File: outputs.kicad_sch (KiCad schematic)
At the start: 33 parts, among them J12 Water_Pump, J13 Fan_Continous, J2 mist, J3 Led, J8 Fan_Exhaust, Q1 AO3406, Q2 AO3406, Q3 AO3406, Q4 AO3406, Q5 AO3406, Q6 AO3406

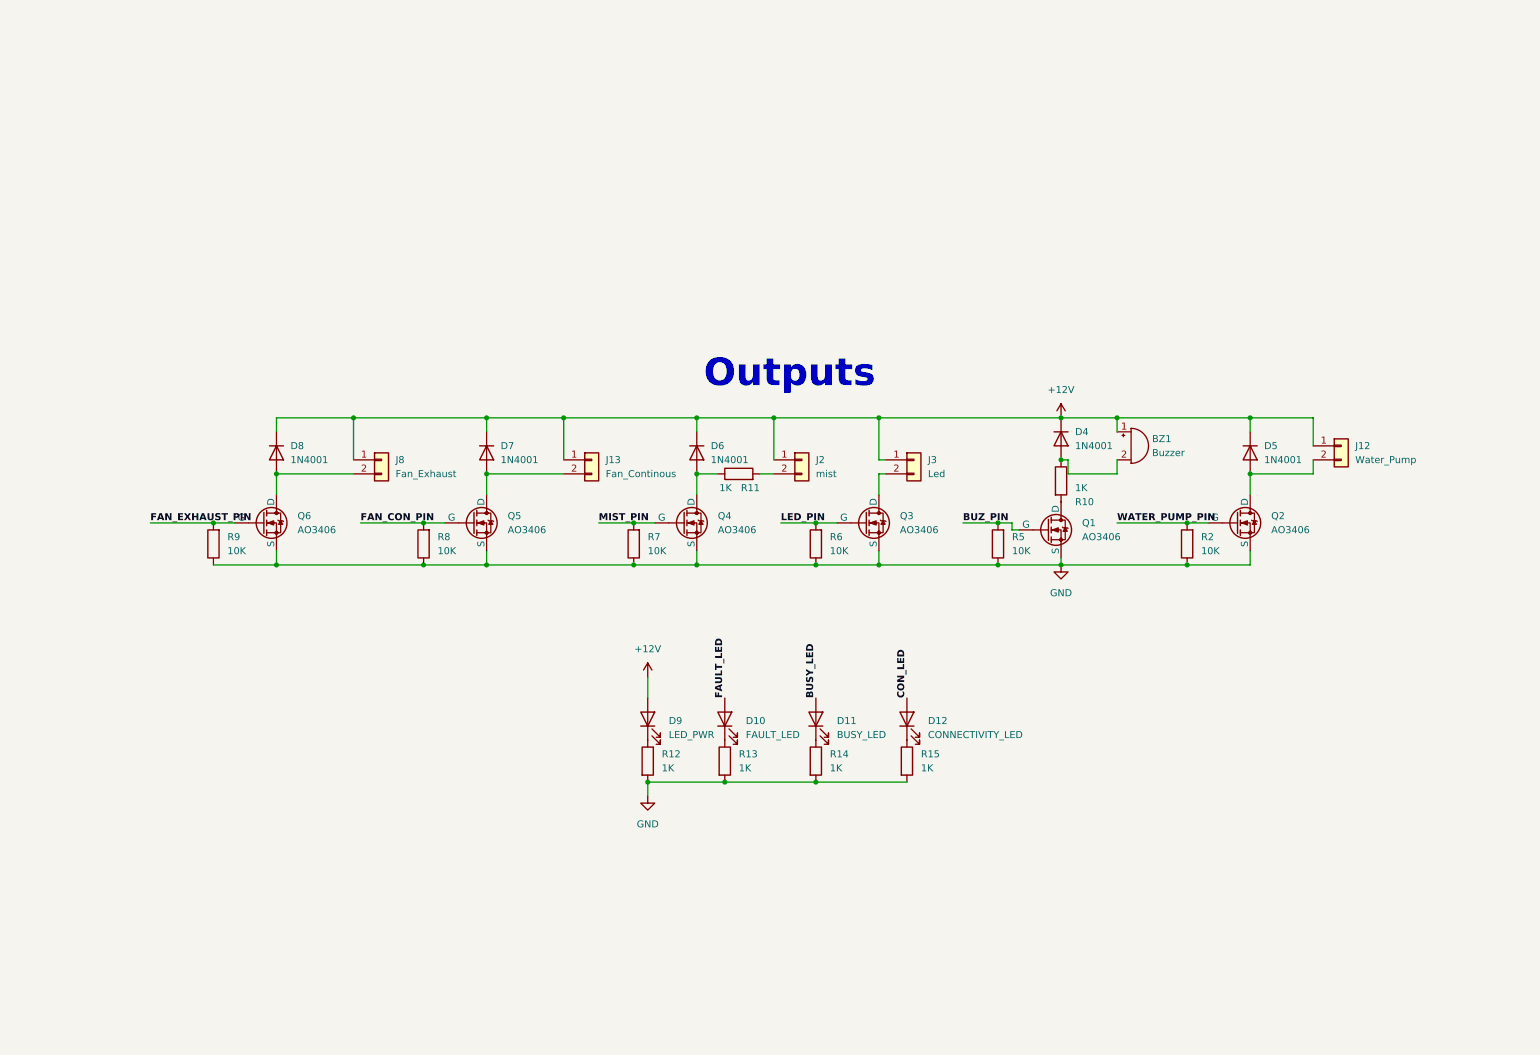
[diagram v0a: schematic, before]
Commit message: Schematic Completed
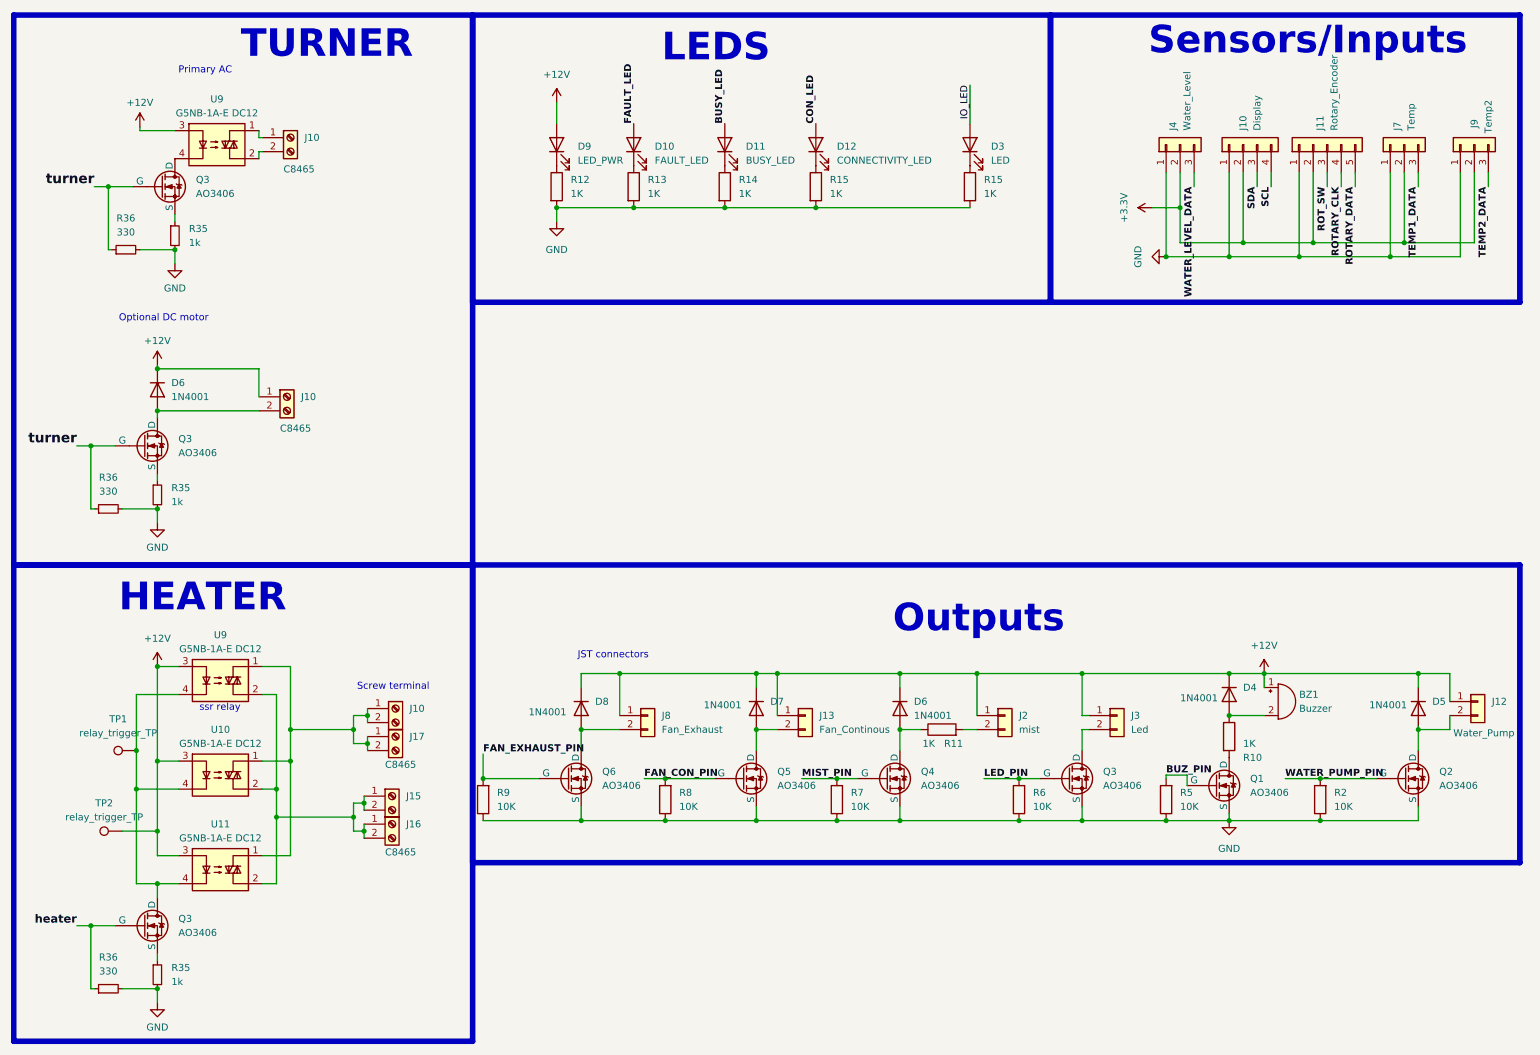
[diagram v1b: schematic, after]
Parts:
- removed R15: 1K, symbol Device:R
- added D3: LED, symbol Device:LED
- added D6: 1N4001, Diode_THT:D_DO-41_SOD81_P10.16mm_Horizontal, symbol Diode:1N4001
- added J10 (x3), J15: C8465, symbol Connector:Screw_Terminal_01x02
- added J10: Display, symbol Connector_Generic:Conn_01x04
- added J11: Rotary_Encoder, symbol Connector_Generic:Conn_01x05
- added J16, J17: Screw_Terminal_01x02, symbol Connector:Screw_Terminal_01x02
- added J4: Water_Level, symbol Connector_Generic:Conn_01x03
- added J7: Temp, symbol Connector_Generic:Conn_01x03
- added J9: Temp2, symbol Connector_Generic:Conn_01x03
- added Q3 (x3): AO3406, symbol Simulation_SPICE:NMOS
- added R15 (x2): 1K, symbol Device:R
- added R35 (x3): 1k, symbol Device:R_Small
- added R36 (x3): 330, symbol Device:R_Small
- added TP1, TP2: relay_trigger_TP, Connector_PinHeader_2.54mm:PinHeader_1x01_P2.54mm_Horizontal, symbol Connector:TestPoint
- added U10, U11, U9 (x2): G5NB-1A-E DC12, Package_SIP:SIP4_Sharp-SSR_P7.62mm_Straight, symbol Relay_SolidState:S102S01
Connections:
- net +12V: now also D6.1 (K), J10.1 (Pin_1), TP2.1, U10.3, U11.3, U9.3, U9.3
- net GND: now also J10.1 (Pin_1), J11.1 (Pin_1), J4.1 (Pin_1), J7.1 (Pin_1), J9.1 (Pin_1), R15.2, R15.2, R35.2, R35.2, R35.2, R36.2, R36.2, R36.2
- net at D12.1 (K): now also R15.1
- new net: J10.1 (Pin_1), J10.2 (Pin_2), J17.1 (Pin_1), J17.2 (Pin_2), U10.1, U11.1, U9.1
- new net: Q3.3 (S), R35.1 (x3)
- new net: J15.1 (Pin_1), J15.2 (Pin_2), J16.1 (Pin_1), J16.2 (Pin_2), U10.2, U11.2, U9.2
- new net: Q3.1 (D), TP1.1, U10.4, U11.4, U9.4
- new net: D3.1 (K), R15.1
- new net: J10.1 (Pin_1), U9.1
- new net: J10.2 (Pin_2), U9.2
- new net: D6.2 (A), J10.2 (Pin_2), Q3.1 (D)
- new net: Q3.1 (D), U9.4
- new net +3.3V: J10.2 (Pin_2), J11.2 (Pin_2), J4.2 (Pin_2), J7.2 (Pin_2), J9.2 (Pin_2)
- new net IO_LED: D3.2 (A)
- new net ROTARY_CLK: J11.4 (Pin_4)
- new net ROTARY_DATA: J11.5 (Pin_5)
- new net ROT_SW: J11.3 (Pin_3)
- new net SCL: J10.4 (Pin_4)
- new net SDA: J10.3 (Pin_3)
- new net TEMP1_DATA: J7.3 (Pin_3)
- new net TEMP2_DATA: J9.3 (Pin_3)
- new net WATER_LEVEL_DATA: J4.3 (Pin_3)
- new net heater: Q3.2 (G), R36.1
- new net turner: Q3.2 (G), Q3.2 (G), R36.1, R36.1
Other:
- note added: "HEATER"
- note added: "JST connectors"
- note added: "LEDS"
- note added: "Optional DC motor"
- note added: "Primary AC"
- note added: "Screw terminal"
- note added: "Sensors/Inputs"
- note added: "TURNER"
- note added: "ssr relay"
- moved on the sheet: BZ1, D4, D5, D6, D7, D8, J12, J13, J2, J3, J8, Q1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
